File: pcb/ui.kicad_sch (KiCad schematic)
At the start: 8 parts, among them Q1 BSS84, Q10 BSS84, Q11 2N7002, Q12 BSS84, Q9 BSS84, U18 74LVC1G139, U20 NHD-C12864A1Z-FSW-FBW-HTT

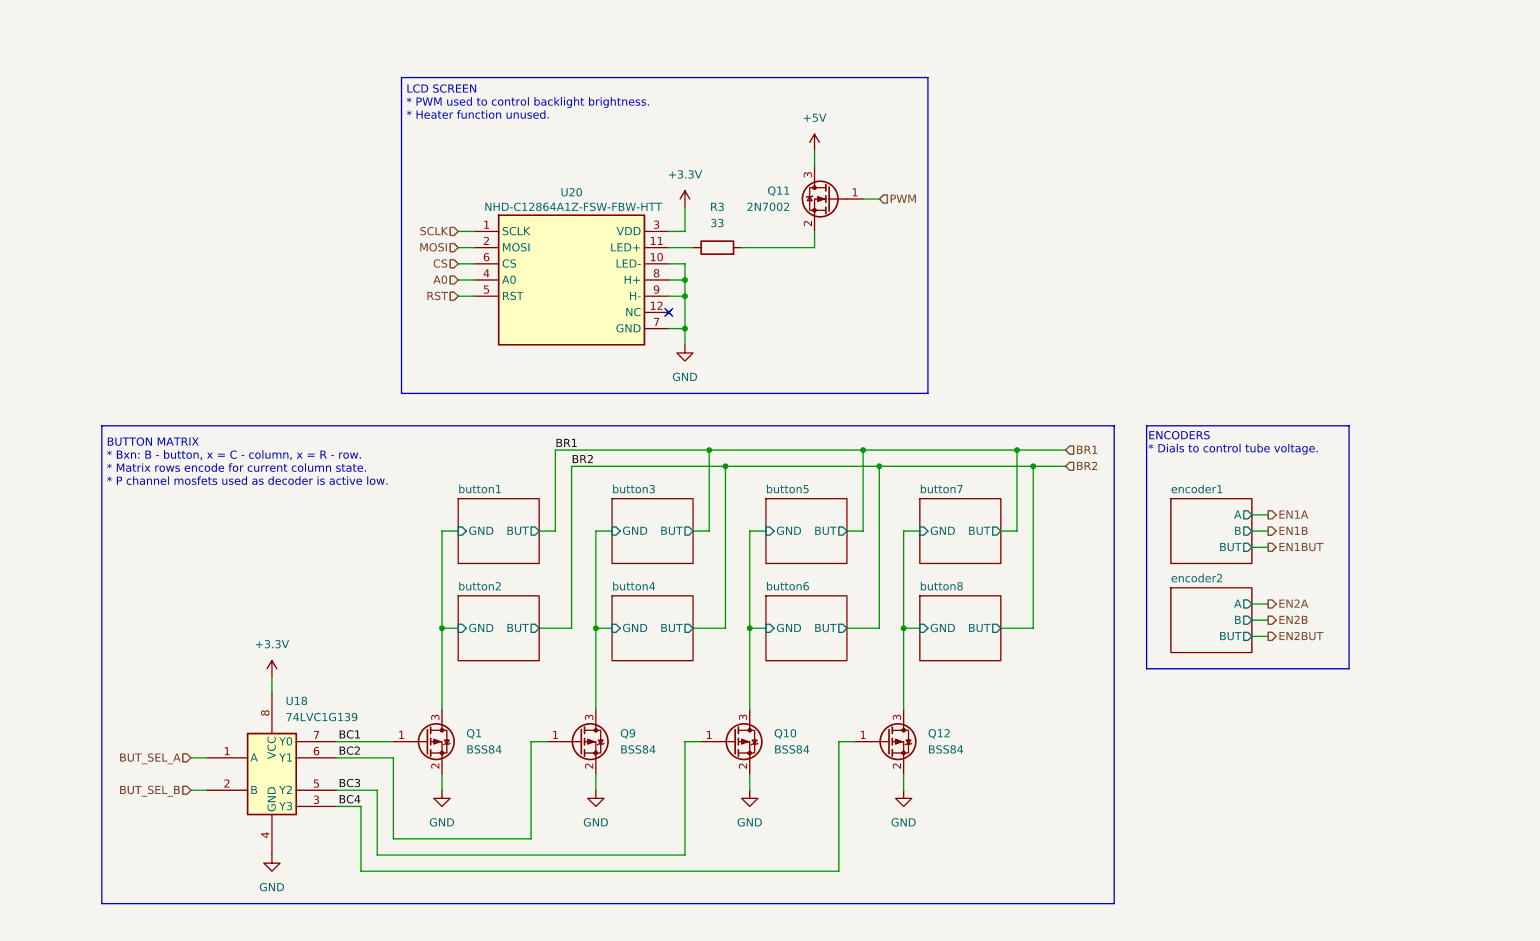
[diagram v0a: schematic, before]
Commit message: chore: many changes checkpoint
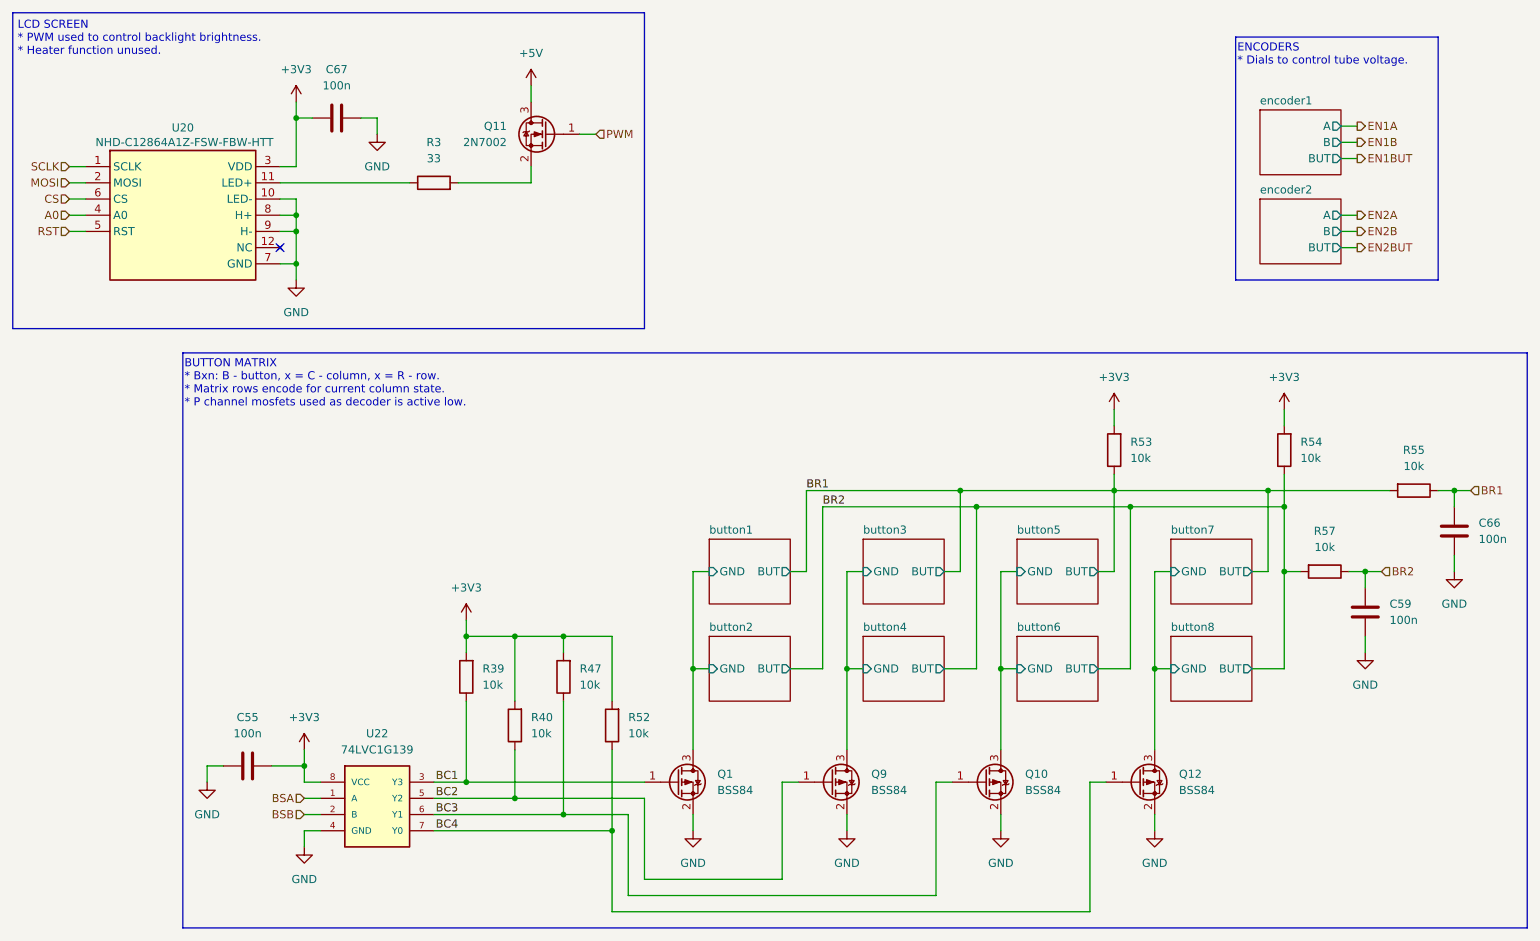
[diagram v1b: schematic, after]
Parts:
- removed U18: 74LVC1G139, symbol 74xGxx:74LVC1G139
- added C55, C67: 100n, Capacitor_SMD:C_0603_1608Metric, symbol Device:C
- added C59, C66: 100n, Capacitor_SMD:C_0201_0603Metric, symbol Device:C
- added R39, R40, R47, R52, R53, R54, R55, R57: 10k, Resistor_SMD:R_0603_1608Metric, symbol Device:R
- added U22: 74LVC1G139, Package_SO:VSSOP-8_2.3x2mm_P0.5mm, symbol project_library:74LVC1G139
- R3: footprint (none) -> Resistor_SMD:R_0603_1608Metric
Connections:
- net BC1: now also R39.1, U22.3 (Y3)
- net BC2: now also R40.1, U22.5 (Y2)
- net BC3: now also R47.1, U22.6 (Y1)
- net BC4: now also R52.1, U22.7 (Y0)
- net BR1: now also C66.2, R53.1, R55.1, R55.2
- net BR2: now also C59.2, R54.1, R57.1, R57.2
- net GND: now also C55.1, C59.1, C66.1, C67.2, U22.4 (GND)
- net +3.3V renamed +3V3
- net +3V3: now also C55.2, C67.1, R39.2, R40.2, R47.2, R52.2, R53.2, R54.2, U22.8 (VCC)
- new net BSA: U22.1 (A)
- new net BSB: U22.2 (B)
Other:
- moved on the sheet: Q1, Q10, Q11, Q12, Q9, R3, U20
